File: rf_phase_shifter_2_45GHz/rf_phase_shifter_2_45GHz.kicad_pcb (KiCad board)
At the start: 2 copper layers, 12 parts, among them J1 Conn_Coaxial, J2 Conn_Coaxial, J3 Conn_Coaxial

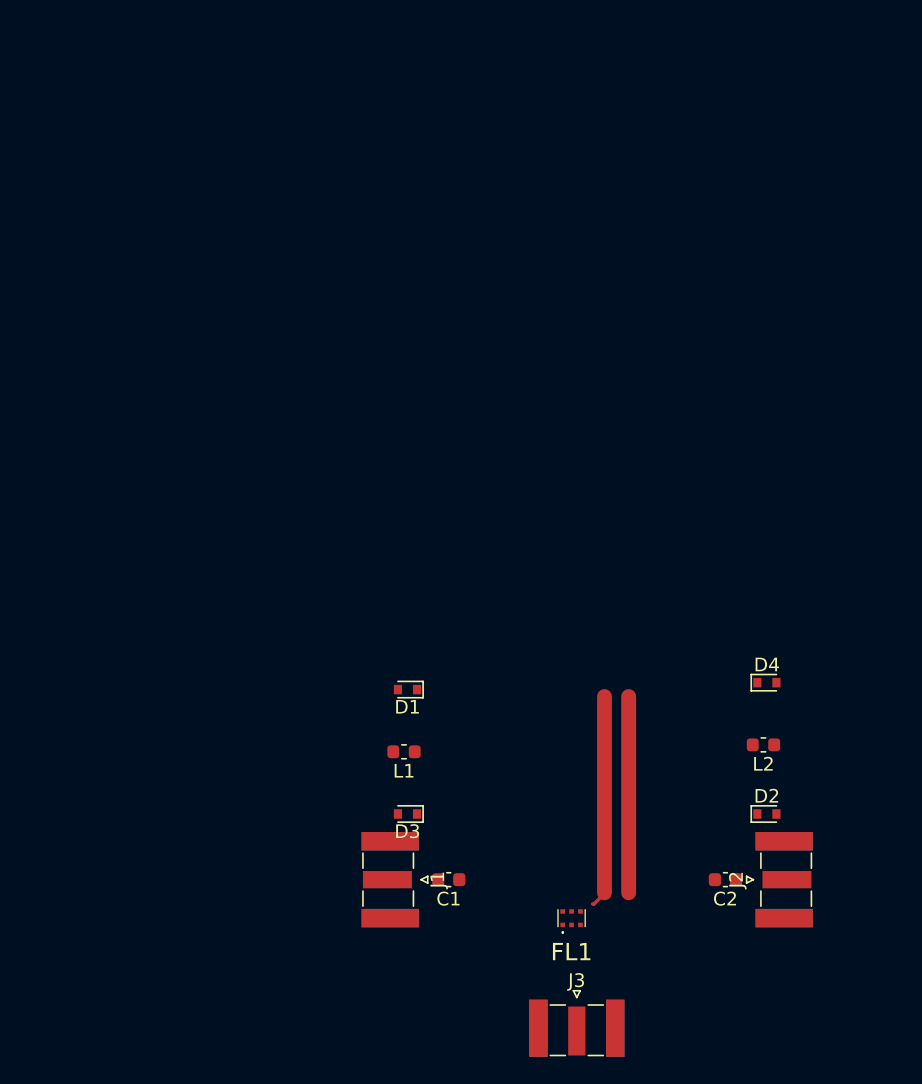
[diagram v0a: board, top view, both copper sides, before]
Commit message: updated libs
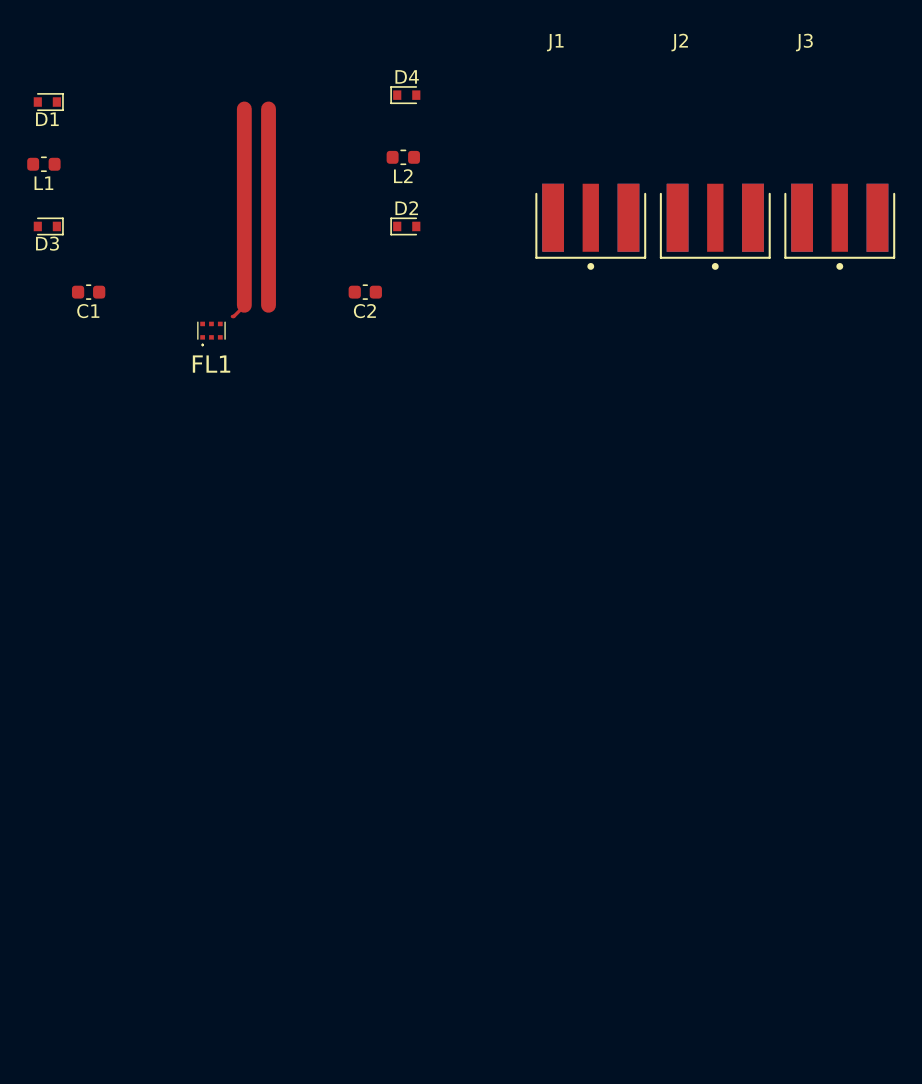
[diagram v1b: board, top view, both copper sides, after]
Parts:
- J1, J2, J3: value Conn_Coaxial -> CON-SMA-EDGE-S; footprint Connector_Coaxial:SMA_Samtec_SMA-J-P-X-ST-EM1_EdgeMount -> analog_rf_phase_shifter_module:CON-SMA-EDGE-S
- moved J3 69.6 mm to (122.7, 36.8)
- moved J1 57.8 mm to (104.4, 36.8), turned to 0 degrees
- moved J2 56.1 mm to (113.6, 36.8), turned to 0 degrees
- moved D3 50.6 mm to (64.5, 44.7)
- moved D1 50.6 mm to (64.5, 35.6)
- moved D2 50.6 mm to (90.9, 44.7)
- moved D4 50.6 mm to (90.9, 35.1)
- moved FL1 50.6 mm to (76.5, 52.4)
- moved L1 50.6 mm to (64.2, 40.1)
- moved L2 50.6 mm to (90.6, 39.6)
- moved C1 50.6 mm to (67.5, 49.5)
- moved C2 50.6 mm to (87.8, 49.5)
